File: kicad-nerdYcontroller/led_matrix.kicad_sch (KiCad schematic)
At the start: 50 parts

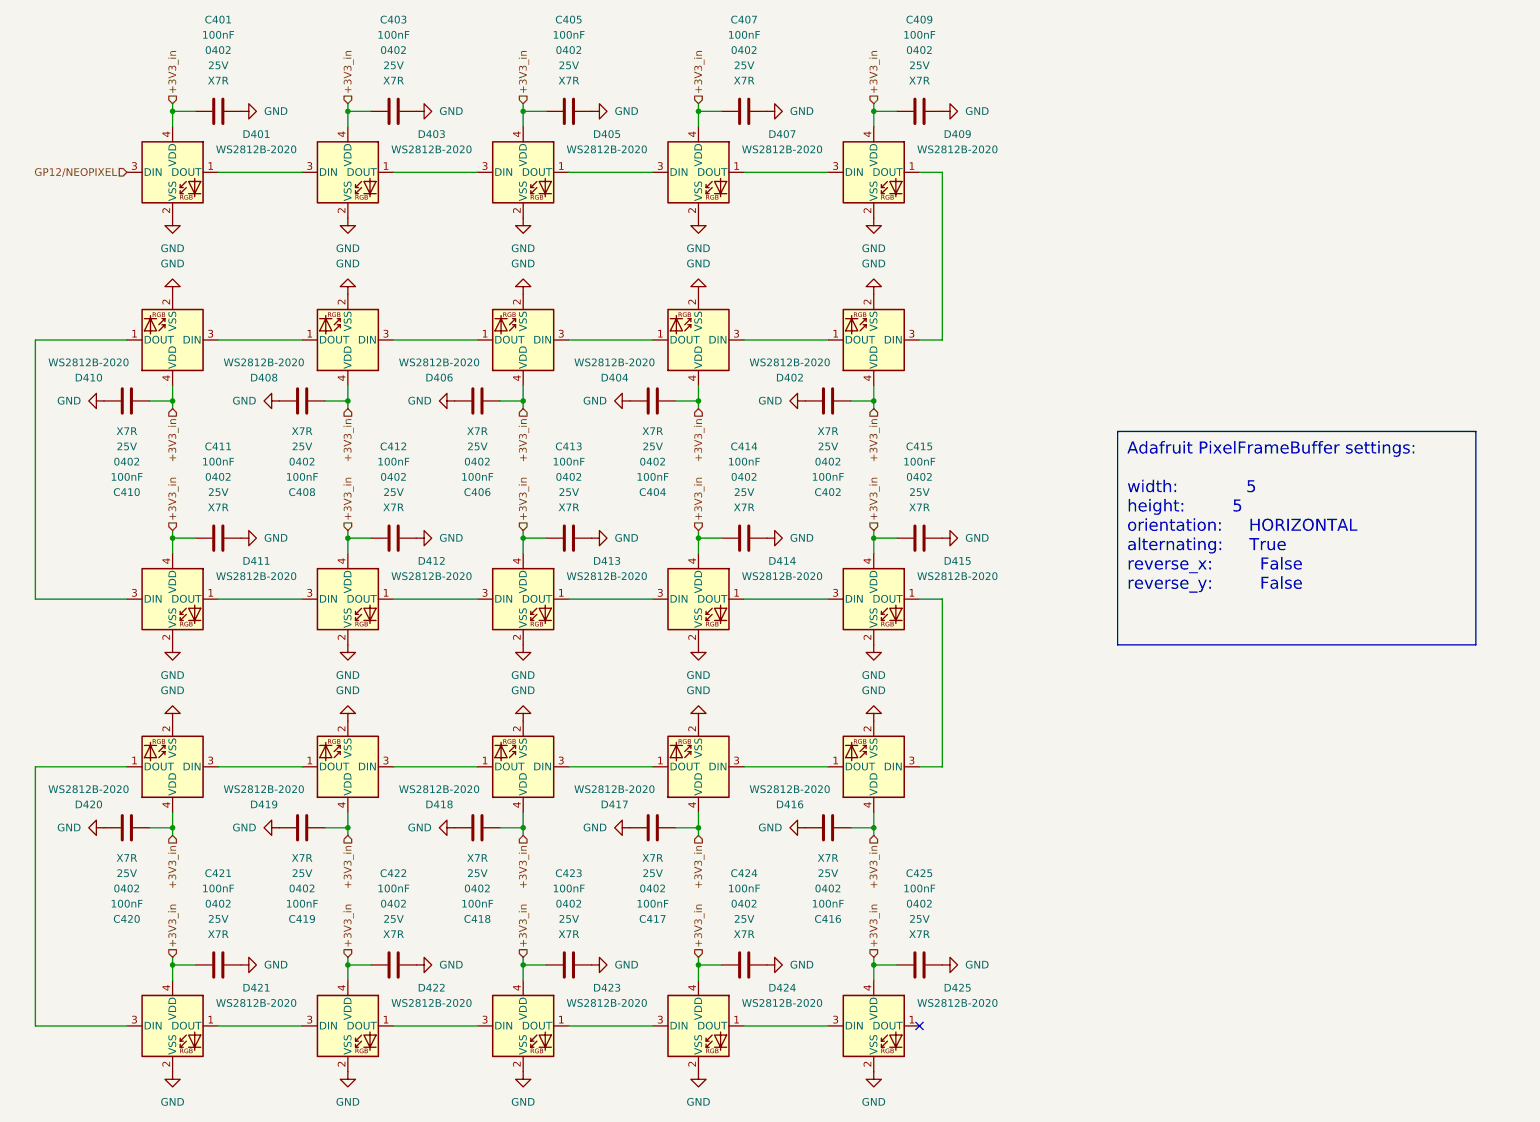
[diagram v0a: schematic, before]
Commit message: Adding KiCad files for first controller production.
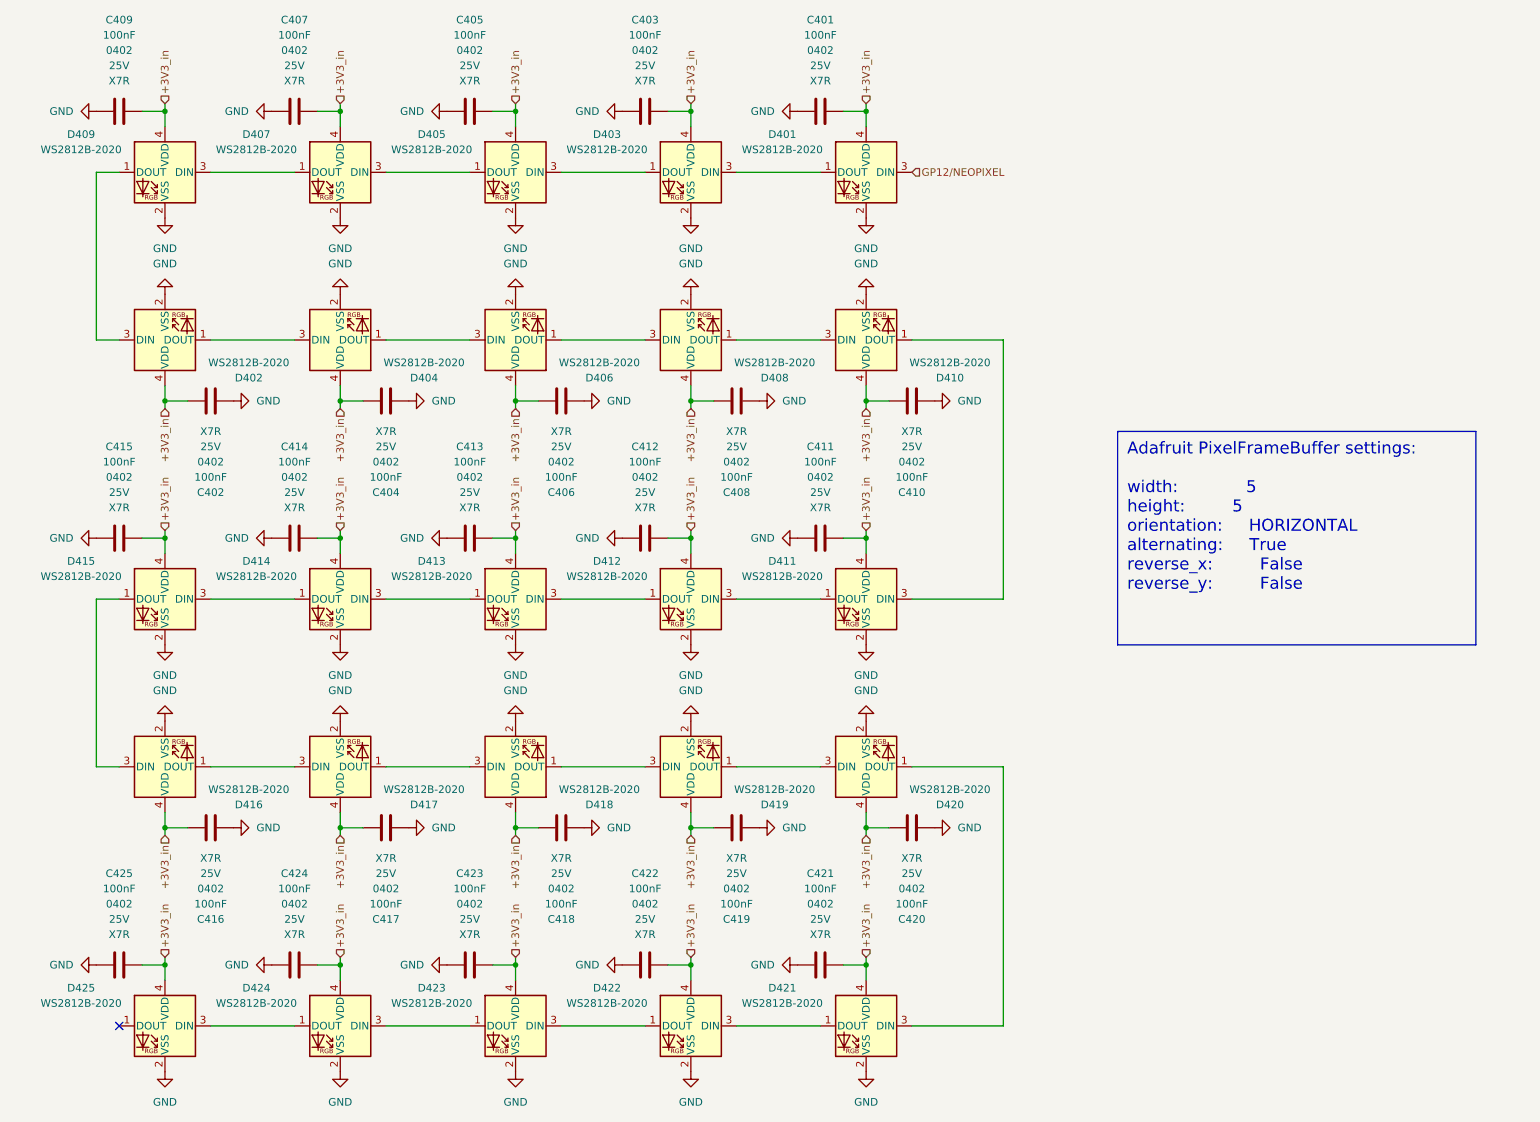
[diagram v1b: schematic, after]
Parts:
- D401, D402, D403, D404, D405, D406, D407, D408, D409, D410, D411, D412, D413, D414, D415, D416, D417, D418, D419, D420, D421, D422, D423, D424, D425: footprint LED_SMD:LED_WS2812B-2020_PLCC4_2.0x2.0mm -> kidslab:LED_WS2812B-2020_PLCC4_2.0x2.0mm
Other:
- moved on the sheet: C401, C402, C403, C404, C405, C406, C407, C408, C409, C410, C411, C412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
